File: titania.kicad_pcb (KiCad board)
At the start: 2 copper layers, 83.8 x 40.6 mm, 27 parts, among them P1 CONN_01X16, P2 CONN_01X16, P3 CONN_01X16, P4 CONN_01X16, P5 CONN_01X06, P6 USB_OTG, SW1 SW_PUSH, U1 LD1117S33TR, U2 PIC24FJ1024GB610, Y1 Crystal

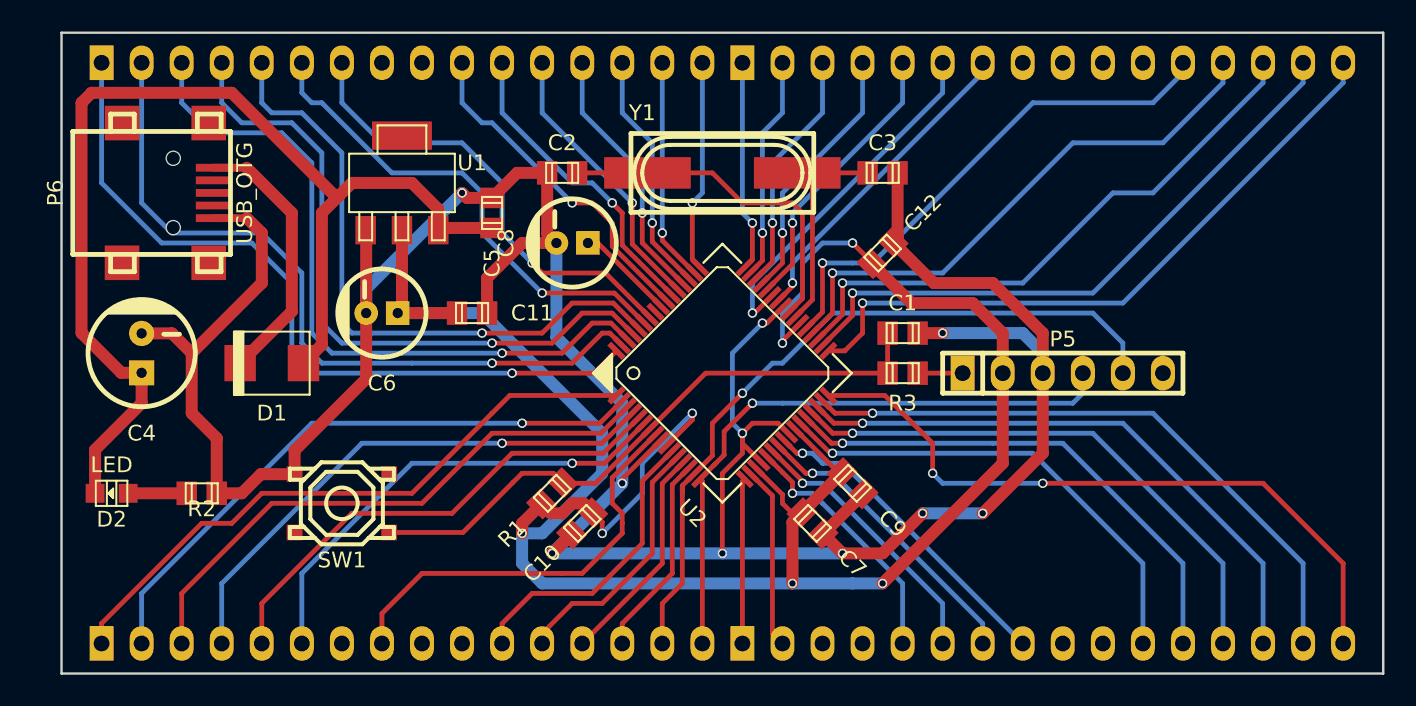
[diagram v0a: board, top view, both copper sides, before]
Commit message: usb host
Signed-off-by: cuki2 <mauricio@krebs.com.br>
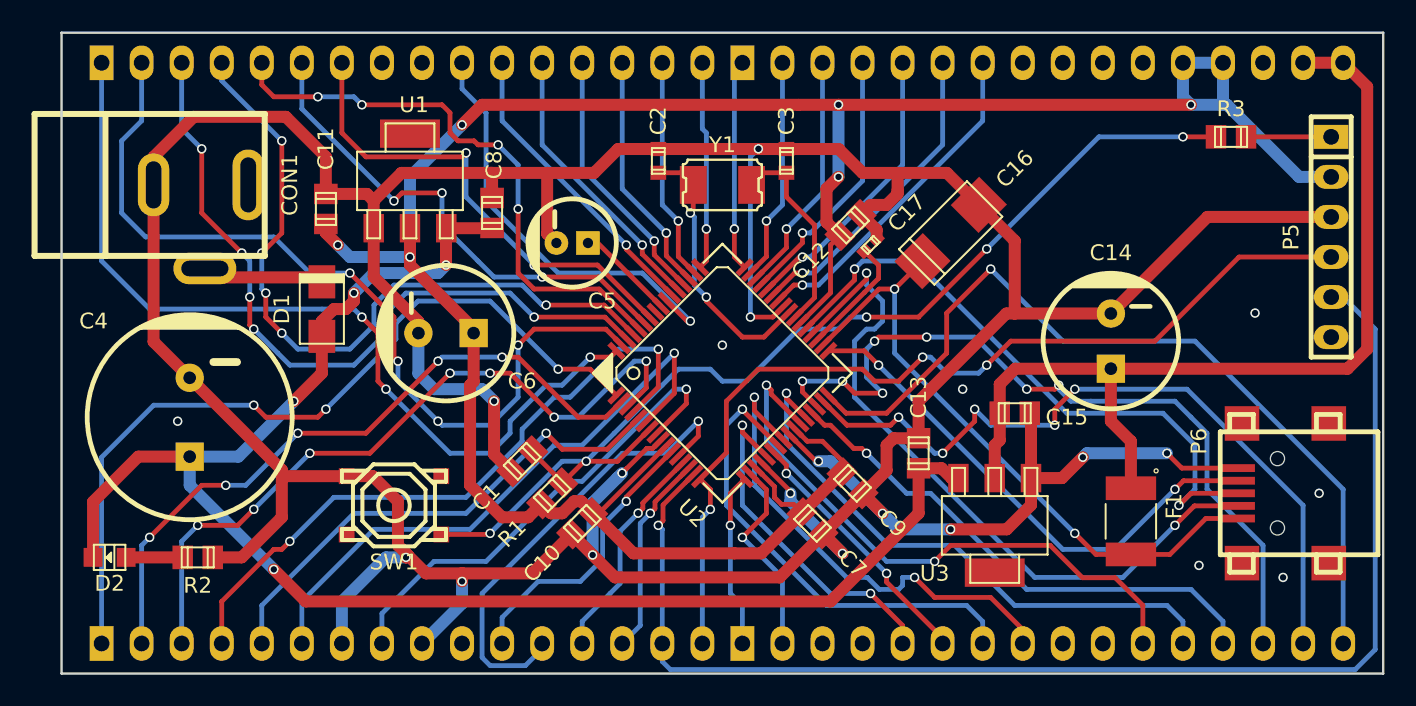
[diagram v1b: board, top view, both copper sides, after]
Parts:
- added C13: 100nF, w_smd_cap:c_0805, F.Cu at (125.5, 64.8)
- added C14: 470uF 16V, w_capacitors:CP_8x11.5mm, F.Cu at (137.7, 57.7)
- added C15: 100nF, w_smd_cap:c_0805, F.Cu at (131.6, 62.2)
- added C16: 150uF 6.3V, w_smd_cap:c_tant_C, F.Cu at (127.5, 50.8)
- added C17: 0.1uF 3.3V, w_smd_cap:c_0402, F.Cu at (122.4, 51.6)
- added CON1: BARREL_JACK, w_conn_misc:dc_socket, F.Cu at (76.7, 47.8)
- added F1: F_Small, MF-MSMF050-2:FUSM4632X85, F.Cu at (138.9, 69.1)
- added U3: LD1117S50TR, w_smd_trans:sot223, F.Cu at (130.3, 69.3)
- C2, C3: footprint w_smd_cap:c_0805 -> w_smd_cap:c_0603
- C4: value 470uF 25V -> 470uF 50V; footprint w_capacitors:CP_6.3x7mm -> w_capacitors:CP_12.5x15mm
- C6: footprint w_capacitors:CP_5x7mm -> w_capacitors:CP_8x11.5mm
- D1: footprint w_smd_diode:do214aa -> w_smd_diode:do214ac
- Y1: footprint w_crystal:crystal_hc-49%2fsmd -> w_crystal:crystal_smd_5x3.2mm
- moved P6 75.2 mm to (149.6, 67.3), turned to 90 degrees
- moved R3 25.7 mm to (145.3, 44.7)
- moved C1 25.5 mm to (100.3, 65.3), turned to 45 degrees
- moved P5 19.1 mm to (151.6, 51.1), turned to 270 degrees
- moved C11 11.4 mm to (87.9, 49.3), turned to 270 degrees
- moved C3 6.14 mm to (117.1, 46.2), turned to 270 degrees
- moved C2 6.14 mm to (109.0, 46.2), turned to 270 degrees
- moved C4 5.08 mm to (79.2, 62.5)
- moved D1 4.67 mm to (87.6, 55.6), turned to 90 degrees
- moved C6 4.26 mm to (95.5, 57.1)
- moved R2 4.07 mm to (79.8, 71.4)
- moved D2 4.07 mm to (74.2, 71.4)
- moved SW1 3.30 mm to (92.2, 68.1)
- moved C12 2.70 mm to (121.2, 50.3)
- moved Y1 0.76 mm to (113.0, 47.8)
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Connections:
- net Net-(C4-Pad1) renamed VCC
- D1 pad 2: Net-(D1-Pad2) -> Net-(CON1-Pad1)
- P1 pad 7: /L7 -> GND
- P1 pad 9: /L9 -> GND
- P4 pad 12: /L37 -> +3.3V
- P4 pad 13: /L36 -> +3.3V
- P4 pad 14: /L35 -> Net-(P4-Pad14)
- P4 pad 15: /L34 -> +5V
- P4 pad 16: /L33 -> +5V
- P6 pad 1: Net-(D1-Pad2) -> /L34
- P6 pad 2: Net-(P6-Pad2) -> /L36
- P6 pad 3: Net-(P6-Pad3) -> /L37
- P6 pad 4: Net-(P6-Pad4) -> /L33
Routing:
- net GND: track 203.0 -> 306.2 mm, vias 10 -> 14
- net +5V: track 0.00 -> 59.7 mm
- net /L15: track 47.4 -> 83.2 mm
- net /MCLR: track 38.9 -> 70.1 mm, vias 0 -> 5
- net /L35: track 37.5 -> 7.60 mm, vias 1 -> 0
- net VCC: track 71.2 -> 98.7 mm, vias 0 -> 4
- net /L16: track 39.3 -> 60.2 mm, vias 1 -> 3
- net +3.3V: track 139.4 -> 160.1 mm, vias 7 -> 6
- net Net-(D1-Pad2): track 17.1 -> 0.00 mm
- net /L12: track 16.5 -> 29.9 mm, vias 0 -> 1
- net /L30: track 37.5 -> 50.2 mm, vias 1 -> 7
- net /L1: track 39.9 -> 52.3 mm, vias 0 -> 3
- net /L23: track 18.9 -> 30.5 mm
- net /L24: track 20.5 -> 31.7 mm, vias 1 -> 2
- net /L32: track 43.3 -> 54.0 mm, vias 2 -> 1
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- added copper zone on B.Cu, net GND
- added copper zone on F.Cu, net GND
